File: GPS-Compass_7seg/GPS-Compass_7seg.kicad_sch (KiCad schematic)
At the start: 8 parts, among them J2 FFC2B28-12-G, U1 OSK3056A-LR, U2 MAX7219

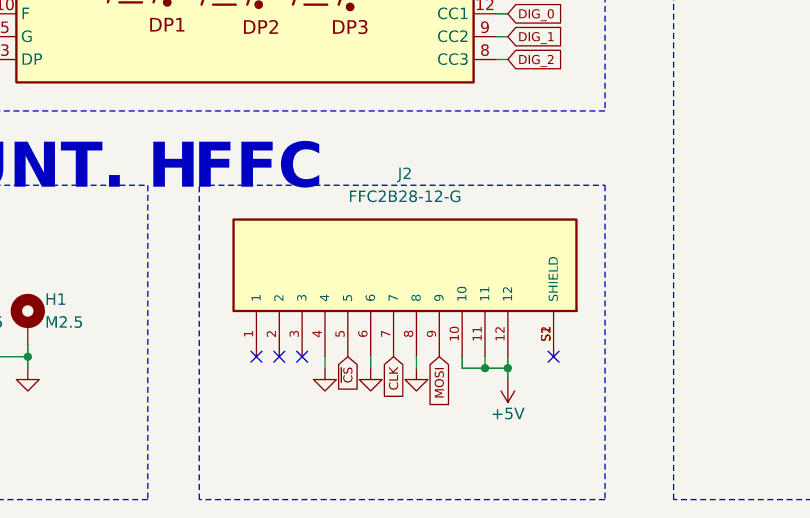
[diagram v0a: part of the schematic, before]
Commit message: GPS Compass - schematic
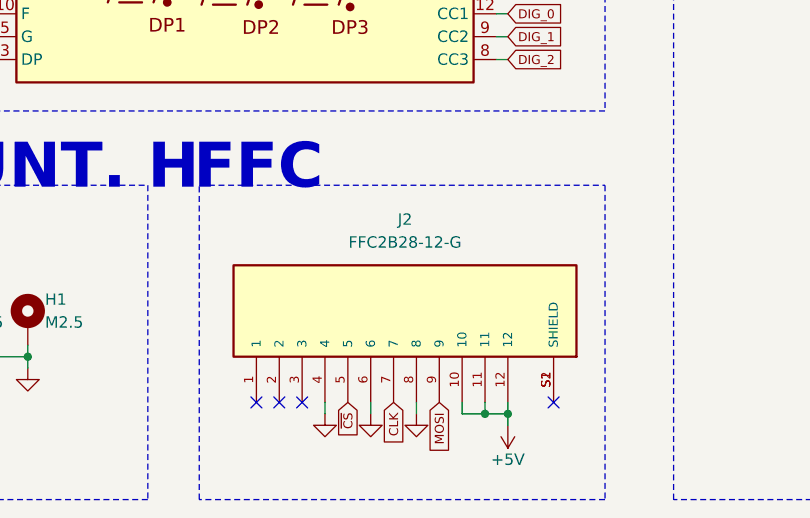
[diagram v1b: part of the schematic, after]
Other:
- moved on the sheet: J2
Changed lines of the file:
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@@
 	)
 	(junction
-		(at 125.73 118.11)
+		(at 125.73 123.19)
 		(diameter 0)
 		(color 0 0 0 0)
 	)
 	(junction
-		(at 123.19 118.11)
+		(at 123.19 123.19)
 		(diameter 0)
 		(color 0 0 0 0)
@@
 	)
 	(no_connect
-		(at 97.79 116.84)
+		(at 97.79 121.92)
 	)
 	(no_connect
-		(at 102.87 116.84)
+		(at 102.87 121.92)
 	)
 	(no_connect
@@
 	)
 	(no_connect
-		(at 100.33 116.84)
+		(at 100.33 121.92)
 	)
 	(no_connect
@@
 	)
 	(no_connect
-		(at 130.81 116.84)
+		(at 130.81 121.92)
 	)
 	(no_connect
@@
 	(wire
 		(pts
-			(xy 125.73 118.11) (xy 123.19 118.11)
+			(xy 125.73 123.19) (xy 123.19 123.19)
 		)
 		(stroke
@@
 	(wire
 		(pts
-			(xy 123.19 118.11) (xy 123.19 116.84)
+			(xy 123.19 123.19) (xy 123.19 121.92)
 		)
 		(stroke
@@
 	(wire
 		(pts
-			(xy 110.49 116.84) (xy 110.49 118.11)
+			(xy 110.49 121.92) (xy 110.49 123.19)
 		)
 		(stroke
@@
 	(wire
 		(pts
-			(xy 125.73 119.38) (xy 125.73 118.11)
+			(xy 125.73 124.46) (xy 125.73 123.19)
 		)
 		(stroke
@@
 	(wire
 		(pts
-			(xy 125.73 118.11) (xy 125.73 116.84)
+			(xy 125.73 123.19) (xy 125.73 121.92)
 		)
 		(stroke
@@
 	(wire
 		(pts
-			(xy 115.57 116.84) (xy 115.57 118.11)
+			(xy 115.57 121.92) (xy 115.57 123.19)
 		)
 		(stroke
@@
 	(wire
 		(pts
-			(xy 123.19 118.11) (xy 120.65 118.11)
+			(xy 123.19 123.19) (xy 120.65 123.19)
 		)
 		(stroke
@@
 	(wire
 		(pts
-			(xy 120.65 118.11) (xy 120.65 116.84)
+			(xy 120.65 123.19) (xy 120.65 121.92)
 		)
 		(stroke
@@
 	(wire
 		(pts
-			(xy 105.41 116.84) (xy 105.41 118.11)
+			(xy 105.41 121.92) (xy 105.41 123.19)
 		)
 		(stroke
@@
 			"AAAAAAAAAAAAAAAAAAAAAAAAAAAAAAAAAAAAAAAAAAAAAAAAAAAAAAAAAAAAAAAAAAAAAAAAAAAA"
 			"AAAAAAAAAAAAAAAAAAAAAAAAAAAAAAAAAAAAAAAAAAAAAAAAAAAAAAAAAAAAAAAAAAAAAAAAAAAA"
+			"AAAAAAAAAAAAAAAAAAAAAAAAAAAAAAAAAAAAAAAAAAAAAAAAAAAAAAAAAAAAAAAAAAAAAAAAAAAA"
+			"AAAAAAAAAAAAAAAAAAAAAAAAAAAAAAAAAAAAAAAAAAAAAAAAAAAAAAAAAAAAAAAAAAAAAAAAAAAA"
+			"AAAAAAAAAAAAAAAAAAAAAAAAAAAAAAAAAAAAAAAAAAAAAAAAAAAAAAAAAAAAAAAAAAAAAAAAAAAA"
+			"AAAAAAAAAAAAAAAAAAAAAAAAAAAAAAAAAAAAAAAAAAAAAAAAAAAAAAAAAAAAAAAAAAAAAAAAAAAA"
+			"AAAAAAAAAAAAAAAAAAAAAAAAAAAAAAAAAAAAAAAAAAAAAAAAAAAAAAAAAAAAAAAAAAAAAAAAAAAA"
+			"AAAAAAAAAAAAAAAAAAAAAAAAAAAAAAAAAAAAAAAAAAAAAAAAAAAAAAAAAAAAAAAAAAAAAAAAAAAA"
+			"AAAAAAAAAAAAAAAAAAAAAAAAAAAAAAAAAAAAAAAAAAAAAAAAAAAAAAAAAAAAAAAAAAAAAAAAAAAA"
+			"AAAAAAAAAAAAAAAAAAAAAAAAAAAAAAAAAAAAAAAAAAAAAAAAAAAAAAAAAAAAAAAAAAAAAAAAAAAA"
+			"AAAAAAAAAAAAAAAAAAAAAAAAAAAAAAAAAAAAAAAAAAAAAAAAAAAAAAAAAAAAAAAAAAAAAAAAAAAA"
+			"AAAAAAAAAAAAAAAAAAAAAAAAAAAAAAAAAAAAAAAAAAAAAAAAAAAAAAAAAAAAAAAAAAAAAAAAAAAA"
+			"AAAAAAAAAAAAAAAAAAAAAAAAAAAAAAAAAAAAAAAAAAAAAAAAAAAAAAAAAAAAAAAAAAAAAAAAAAAA"
+			"AAAAAAAAAAAAAAAAAAAAAAAAAAAAAAAAAAAAAAAAAAAAAAAAAAAAAAAAAAAAAAAAAAAAAAAAAAAA"
+			"AAAAAAAAAAAAAAAAAAAAAAAAAAAAAAAAAAAAAAAAAAAAAAAAAAAAAAAAAAAAAAAAAAAAAAAAAAAA"
+			"AAAAAAAAAAAAAAAAAAAAAAAAAAAAAAAAAAAAAAAAAAAAAAAAAAAAAAAAAAAAAAAAAAAAAAAAAAAA"
+			"AAAAAAAAAAAAAAAAAAAAAAAAAAAAAAAAAAAAAAAAAAAAAAAAAAAAAAAAAAAAAAAAAAAAAAAAAAAA"
+			"AAAAAAAAAAAAAAAAAAAAAAAAAAAAAAAAAAAAAAAAAAAAAAAAAAAAAAAAAAAAAAAAAAAAAAAAAAAA"
+			"AAAAAAAAAAAAAAAAAAAAAAAAAAAAAAAAAAAAAAAAAAAAAAAAAAAAAAAAAAAAAAAAAAAAAAAAAAAA"
+			"AAAAAAAAAAAAAAAAAAAAAAAAAAAAAAAAAAAAAAAAAAAAAAAAAAAAAAAAAAAAAAAAAAAAAAAAAAAA"
 			"AA=="
 		)
@@
 	(global_label "MOSI"
 		(shape input)
-		(at 118.11 116.84 270)
+		(at 118.11 121.92 270)
 		(fields_autoplaced yes)
 		(effects
@@
 		)
 		(property "Intersheetrefs" "${INTERSHEET_REFS}"
-			(at 118.11 122.2148 90)
+			(at 118.11 127.2948 90)
 			(effects
 				(font
@@
 	(global_label "~{CS}"
 		(shape input)
-		(at 107.95 116.84 270)
+		(at 107.95 121.92 270)
 		(fields_autoplaced yes)
 		(effects
@@
 		)
 		(property "Intersheetrefs" "${INTERSHEET_REFS}"
-			(at 107.95 120.7152 90)
+			(at 107.95 125.7952 90)
 			(effects
 				(font
@@
 	(global_label "CLK"
 		(shape input)
-		(at 113.03 116.84 270)
+		(at 113.03 121.92 270)
 		(fields_autoplaced yes)
 		(effects
@@
 		)
 		(property "Intersheetrefs" "${INTERSHEET_REFS}"
-			(at 113.03 121.5671 90)
+			(at 113.03 126.6471 90)
 			(effects
 				(font
@@
 	(symbol
 		(lib_id "gps-compass_sch:FFC2B28-12-G")
-		(at 113.03 106.68 90)
+		(at 113.03 111.76 90)
 		(unit 1)
 		(exclude_from_sim no)
@@
 		(fields_autoplaced yes)
 		(property "Reference" "J2"
-			(at 114.3 96.52 90)
+			(at 114.3 101.6 90)
 			(effects
 				(font
@@
 		)
 		(property "Value" "FFC2B28-12-G"
-			(at 114.3 99.06 90)
+			(at 114.3 104.14 90)
 			(effects
 				(font
@@
 		)
 		(property "Footprint" "gps-compass_brd:GCT_FFC2B28-12-G"
-			(at 113.03 106.68 0)
+			(at 113.03 111.76 0)
 			(effects
 				(font
@@
 		)
 		(property "Datasheet" "https://cz.mouser.com/ProductDetail/GCT/FFC2B28-12-G?qs=KUoIvG%2F9Ilb3Lmj8zxhxfA%3D%3D"
-			(at 113.03 106.68 0)
+			(at 113.03 111.76 0)
 			(effects
 				(font
@@
 		)
 		(property "Description" ""
-			(at 113.03 106.68 0)
+			(at 113.03 111.76 0)
 			(effects
 				(font
@@
 		)
 		(property "MF" "Global Connector Technology"
-			(at 113.03 106.68 0)
+			(at 113.03 111.76 0)
 			(effects
 				(font
@@
 		)
 		(property "MAXIMUM_PACKAGE_HEIGHT" "1.75mm"
-			(at 113.03 106.68 0)
+			(at 113.03 111.76 0)
 			(effects
 				(font
@@
 		)
 		(property "Package" "None"
-			(at 113.03 106.68 0)
+			(at 113.03 111.76 0)
 			(effects
 				(font
@@
 		)
 		(property "Price" "None"
-			(at 113.03 106.68 0)
+			(at 113.03 111.76 0)
 			(effects
 				(font
@@
 		)
 		(property "Check_prices" "https://www.snapeda.com/parts/FFC2B28-12-G/Global+Connector+Technology/view-part/?ref=eda"
-			(at 113.03 106.68 0)
+			(at 113.03 111.76 0)
 			(effects
 				(font
@@
 		)
 		(property "STANDARD" "Manufacturer Recommendations"
-			(at 113.03 106.68 0)
+			(at 113.03 111.76 0)
 			(effects
 				(font
@@
 		)
 		(property "PARTREV" "A"
-			(at 113.03 106.68 0)
+			(at 113.03 111.76 0)
 			(effects
 				(font
@@
 		)
 		(property "SnapEDA_Link" "https://www.snapeda.com/parts/FFC2B28-12-G/Global+Connector+Technology/view-part/?ref=snap"
-			(at 113.03 106.68 0)
+			(at 113.03 111.76 0)
 			(effects
 				(font
@@
 		)
 		(property "MP" "FFC2B28-12-G"
-			(at 113.03 106.68 0)
+			(at 113.03 111.76 0)
 			(effects
 				(font
@@
 		)
 		(property "Description_1" "12 Position FFC, FPC Connector Contacts, Top and Bottom 0.020 (0.50mm) Surface Mount, Right Angle"
-			(at 113.03 106.68 0)
+			(at 113.03 111.76 0)
 			(effects
 				(font
@@
 		)
 		(property "Availability" "In Stock"
-			(at 113.03 106.68 0)
+			(at 113.03 111.76 0)
 			(effects
 				(font
@@
 		)
 		(property "MANUFACTURER" "GCT"
-			(at 113.03 106.68 0)
+			(at 113.03 111.76 0)
 			(effects
 				(font
@@
 	(symbol
 		(lib_id "power:GND")
-		(at 110.49 118.11 0)
+		(at 110.49 123.19 0)
 		(mirror y)
 		(unit 1)
@@
 		(fields_autoplaced yes)
 		(property "Reference" "#PWR08"
-			(at 110.49 124.46 0)
+			(at 110.49 129.54 0)
 			(effects
 				(font
@@
 		)
 		(property "Value" "GND"
-			(at 110.49 123.19 0)
+			(at 110.49 128.27 0)
 			(effects
 				(font
@@
 		)
 		(property "Footprint" ""
-			(at 110.49 118.11 0)
+			(at 110.49 123.19 0)
 			(effects
 				(font
@@
 		)
 		(property "Datasheet" ""
-			(at 110.49 118.11 0)
+			(at 110.49 123.19 0)
 			(effects
 				(font
@@
 		)
 		(property "Description" ""
-			(at 110.49 118.11 0)
+			(at 110.49 123.19 0)
 			(effects
 				(font
@@
 	(symbol
 		(lib_id "power:GND")
-		(at 115.57 118.11 0)
+		(at 115.57 123.19 0)
 		(mirror y)
 		(unit 1)
@@
 		(fields_autoplaced yes)
 		(property "Reference" "#PWR09"
-			(at 115.57 124.46 0)
+			(at 115.57 129.54 0)
 			(effects
 				(font
@@
 		)
 		(property "Value" "GND"
-			(at 115.57 123.19 0)
+			(at 115.57 128.27 0)
 			(effects
 				(font
@@
 		)
 		(property "Footprint" ""
-			(at 115.57 118.11 0)
+			(at 115.57 123.19 0)
 			(effects
 				(font
@@
 		)
 		(property "Datasheet" ""
-			(at 115.57 118.11 0)
+			(at 115.57 123.19 0)
 			(effects
 				(font
@@
 		)
 		(property "Description" ""
-			(at 115.57 118.11 0)
+			(at 115.57 123.19 0)
 			(effects
 				(font
@@
 	(symbol
 		(lib_id "power:+5V")
-		(at 125.73 119.38 180)
+		(at 125.73 124.46 180)
 		(unit 1)
 		(exclude_from_sim no)
@@
 		(dnp no)
 		(property "Reference" "#PWR03"
-			(at 125.73 115.57 0)
+			(at 125.73 120.65 0)
 			(effects
 				(font
@@
 		)
 		(property "Value" "+5V"
-			(at 125.73 123.19 0)
+			(at 125.73 128.27 0)
 			(effects
 				(font
@@
 		)
 		(property "Footprint" ""
-			(at 125.73 119.38 0)
+			(at 125.73 124.46 0)
 			(effects
 				(font
@@
 		)
 		(property "Datasheet" ""
-			(at 125.73 119.38 0)
+			(at 125.73 124.46 0)
 			(effects
 				(font
@@
 		)
 		(property "Description" "Power symbol creates a global label with name \"+5V\""
-			(at 125.73 119.38 0)
+			(at 125.73 124.46 0)
 			(effects
 				(font
@@
 	(symbol
 		(lib_id "power:GND")
-		(at 105.41 118.11 0)
+		(at 105.41 123.19 0)
 		(mirror y)
 		(unit 1)
@@
 		(fields_autoplaced yes)
 		(property "Reference" "#PWR02"
-			(at 105.41 124.46 0)
+			(at 105.41 129.54 0)
 			(effects
 				(font
@@
 		)
 		(property "Value" "GND"
-			(at 105.41 123.19 0)
+			(at 105.41 128.27 0)
 			(effects
 				(font
@@
 		)
 		(property "Footprint" ""
-			(at 105.41 118.11 0)
+			(at 105.41 123.19 0)
 			(effects
 				(font
@@
 		)
 		(property "Datasheet" ""
-			(at 105.41 118.11 0)
+			(at 105.41 123.19 0)
 			(effects
 				(font
@@
 		)
 		(property "Description" ""
-			(at 105.41 118.11 0)
+			(at 105.41 123.19 0)
 			(effects
 				(font
